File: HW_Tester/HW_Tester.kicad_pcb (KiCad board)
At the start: 4 copper layers, 59 parts, among them J3 011/030/040/05x, J4 001, J5 JDS USB, U1 STM32F303CBTx, U2 AMS1117-3.3, Y1 Crystal

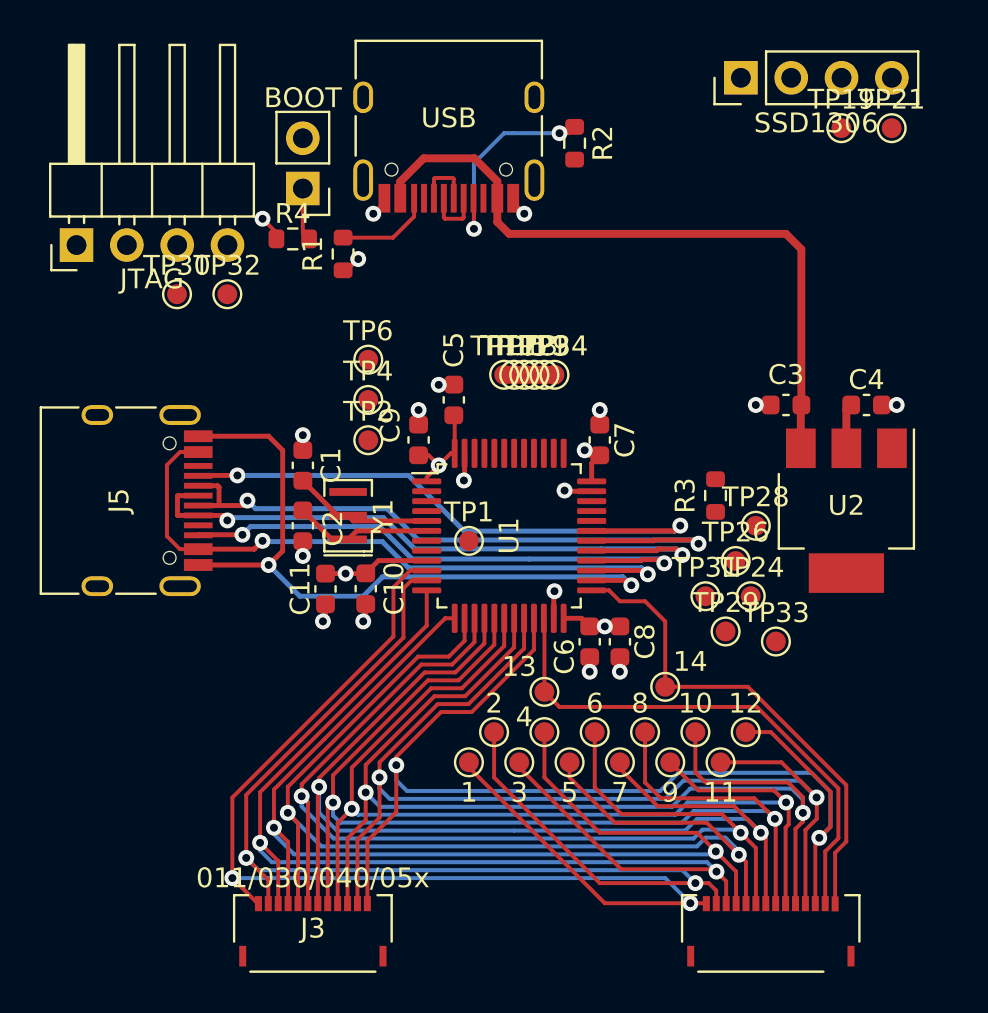
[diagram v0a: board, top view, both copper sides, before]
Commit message: Completed board pending review
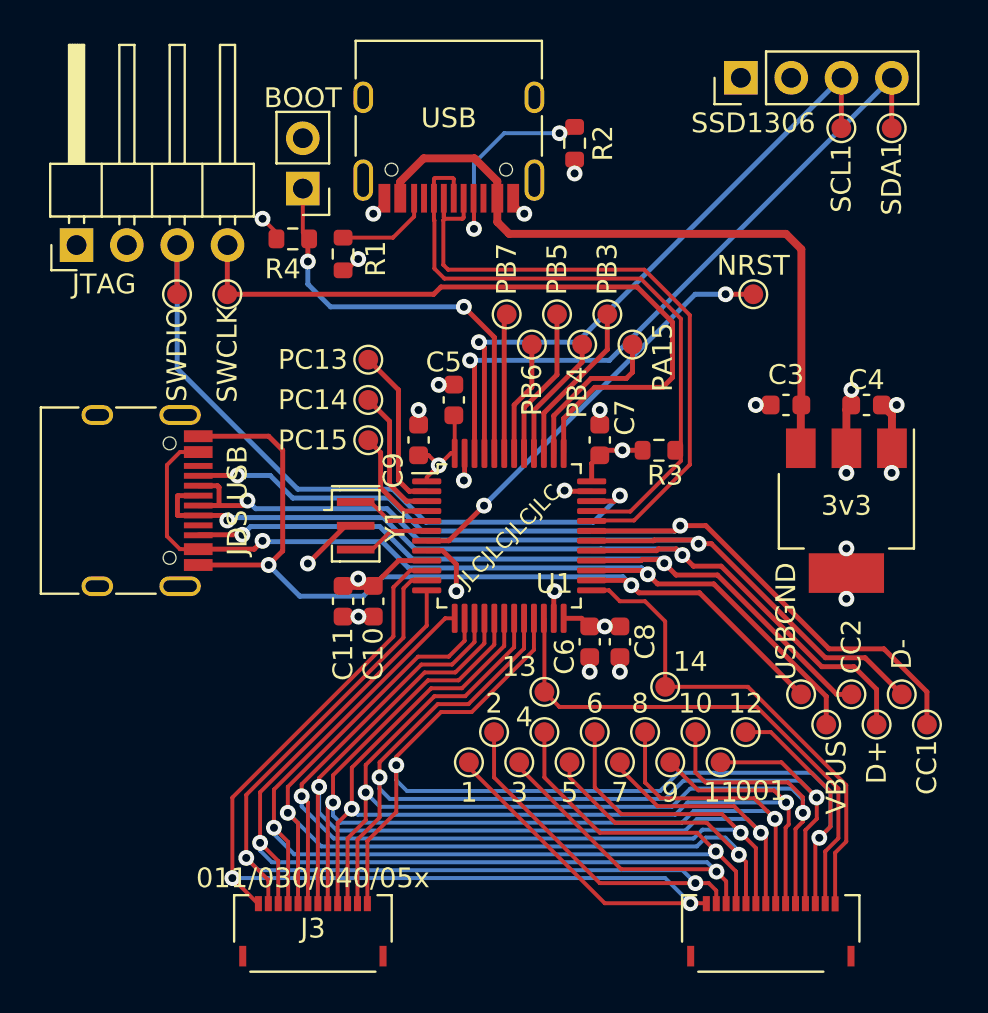
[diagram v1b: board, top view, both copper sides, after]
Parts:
- removed C1, C2: C, Capacitor_SMD:C_0603_1608Metric
- JDS USB: renamed from J5
- Y1: value Crystal -> Resonator
- moved NRST 19.0 mm to (159.6, 69.3)
- moved CC1 13.2 mm to (168.4, 91.1)
- moved D- 10.8 mm to (167.1, 89.5)
- moved D+ 9.07 mm to (165.9, 91.1)
- moved VBUS 8.89 mm to (163.3, 91.1)
- moved USBGND 4.96 mm to (162.1, 89.5)
- moved CC2 4.65 mm to (164.6, 89.5)
- moved PB3 4.40 mm to (152.3, 70.4)
- moved PA15 4.22 mm to (153.5, 71.9)
- moved R3 3.66 mm to (154.9, 77.2), turned to 0 degrees
- moved PB5 3.47 mm to (149.7, 70.4)
- moved PB7 3.05 mm to (147.2, 70.4)
- moved PB4 2.85 mm to (151.0, 71.9)
- moved PB6 1.76 mm to (148.5, 71.9)
- moved C11 1.08 mm to (138.9, 84.8)
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- renumbered U2 to 3v3, TP28 to CC1, TP33 to CC2, TP24 to D+, TP26 to D-, TP1 to NRST, TP34 to PA15, TP9 to PB3, TP11 to PB4, TP13 to PB5, TP15 to PB6, TP17 to PB7, TP6 to PC13, TP4 to PC14, TP2 to PC15, TP19 to SCL1, TP21 to SDA1, TP32 to SWCLK, TP30 to SWDIO, TP29 to USBGND, TP31 to VBUS
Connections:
- U1 pad 5: Net-(C1-Pad2) -> /R+
- U1 pad 6: Net-(C2-Pad2) -> /R-
- U1 pad 8: unconnected-(U1-Pad8) -> GND
- Y1 pad 1: Net-(C2-Pad2) -> /R+
- Y1 pad 2: Net-(C1-Pad2) -> GND
- Y1 pad 3: (no net) -> /R-
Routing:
- net SWCLK-JTCK/I2C1_SDA/UART2_TX: track 0.00 -> 36.7 mm
- net SWDIO_JTMS: track 0.00 -> 36.4 mm, vias 0 -> 1
- net I2C1_SDA/CAN_TX: track 0.00 -> 34.5 mm, vias 0 -> 1
- net I2C1_SCL/CAN_RX: track 0.00 -> 32.1 mm, vias 0 -> 1
- net D-: track 3.00 -> 33.5 mm
- net D+: track 2.99 -> 32.8 mm
- net NRST: track 0.00 -> 21.6 mm, vias 0 -> 2
- net BOOT: track 2.67 -> 21.4 mm, vias 0 -> 2
- net I2C2_SDA/UART1_RX: track 30.2 -> 47.7 mm
- net PA8: track 33.2 -> 47.6 mm
- net I2C2_SCL/UART1_TX: track 34.8 -> 48.2 mm
- net SPI2_MISO/ADC4_IN4: track 33.8 -> 46.7 mm
- net SPI2_MOSI/ADC4_IN5: track 28.3 -> 40.4 mm
- net I2C2_SCK/ADC3_IN5: track 35.9 -> 46.7 mm
- net GND: track 17.2 -> 25.9 mm, vias 18 -> 19
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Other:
- board text added: "JLCJLCJLCJLC"
